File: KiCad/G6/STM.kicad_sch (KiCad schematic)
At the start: 8 parts, among them U12 STM32C051K8T6, Y1 ABS07-32.768KHZ-1-T

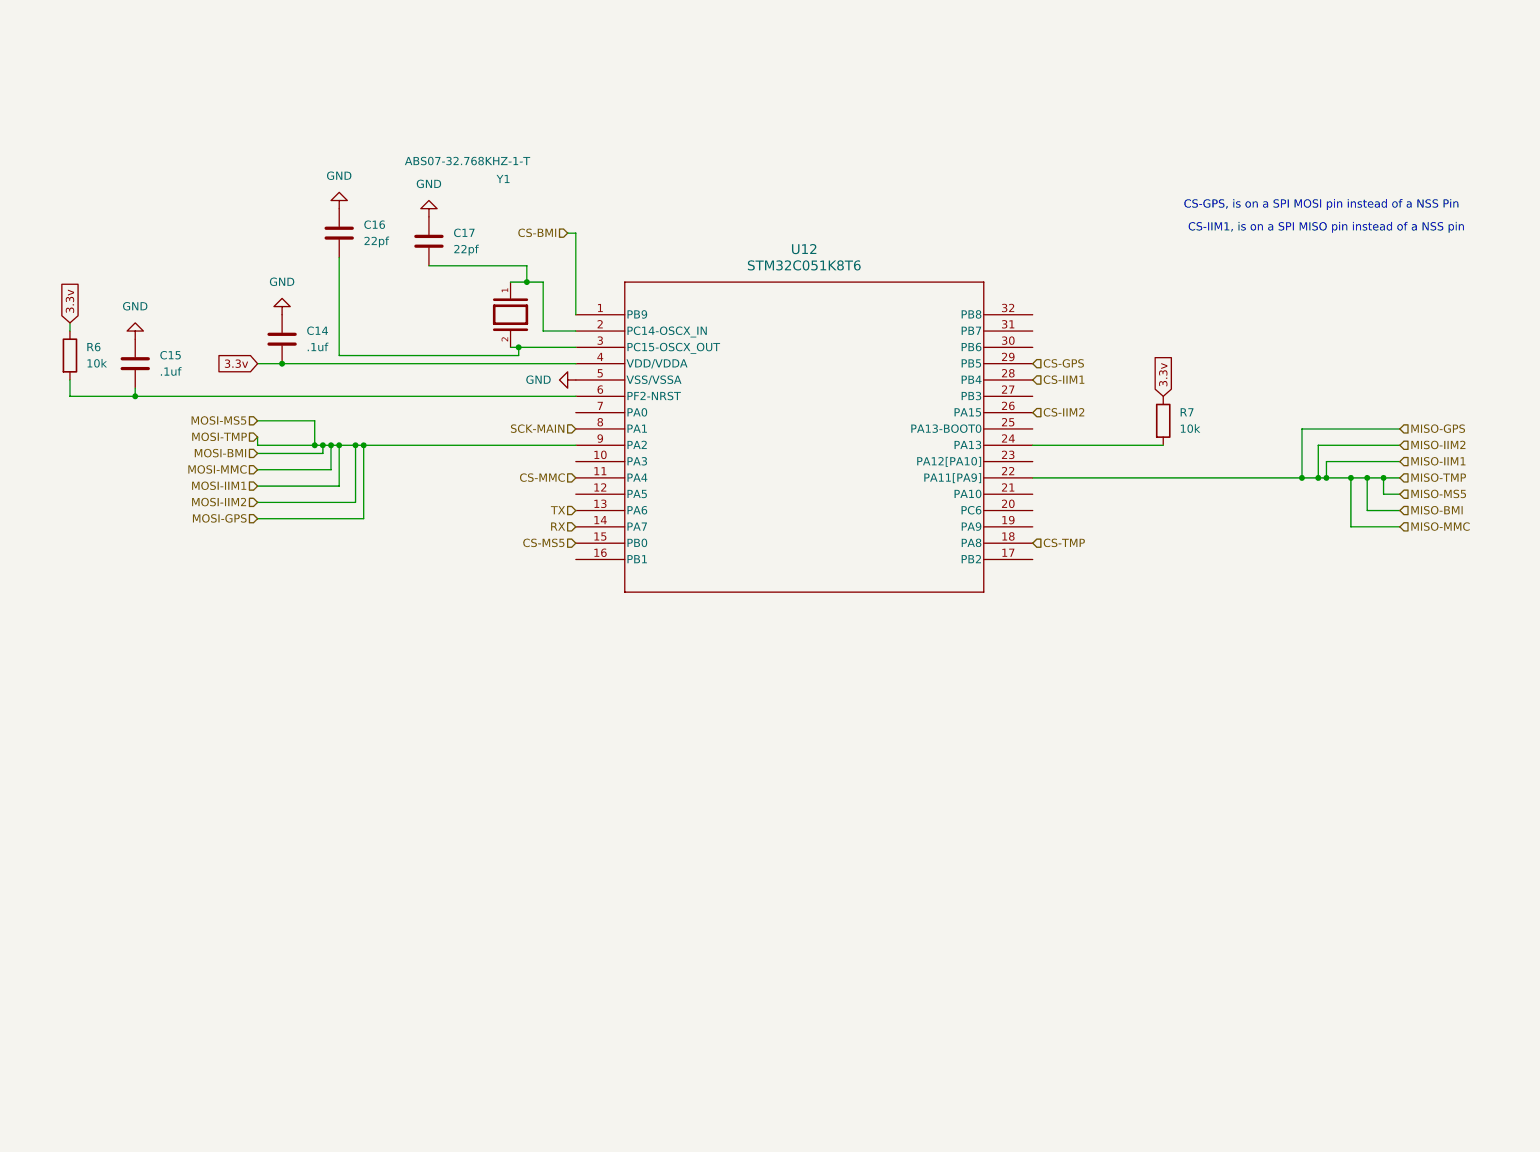
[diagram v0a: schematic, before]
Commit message: g6
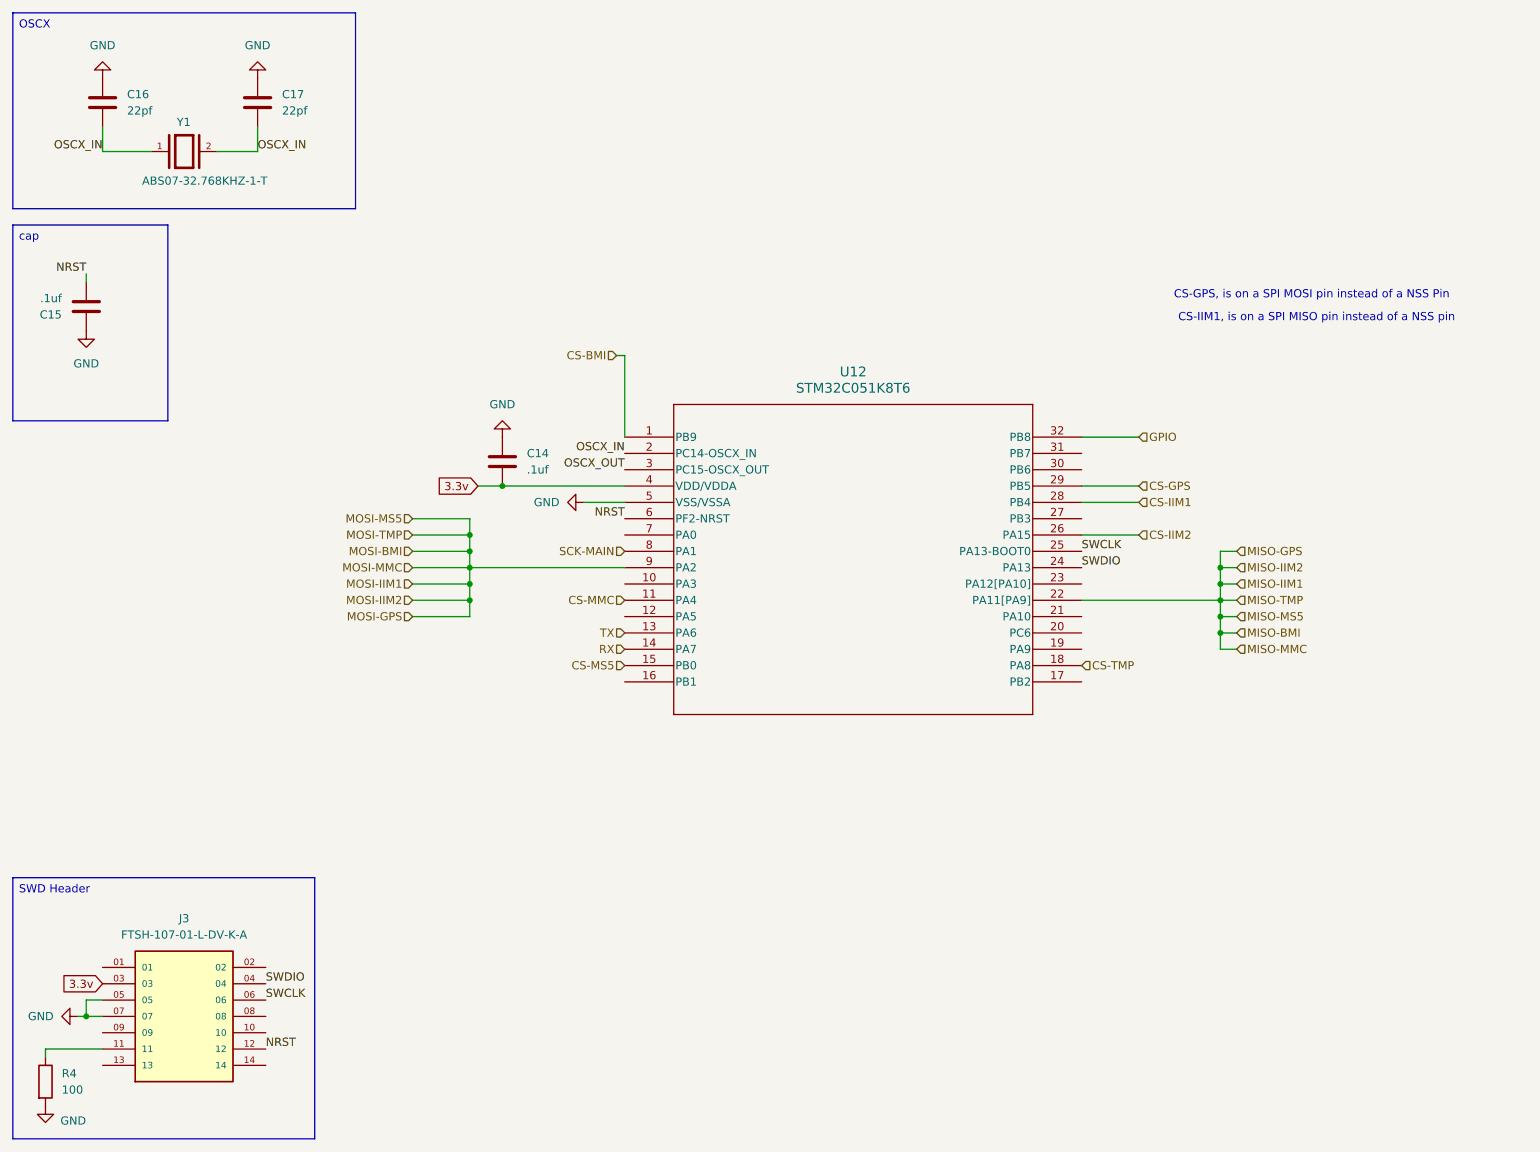
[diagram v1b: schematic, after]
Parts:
- removed R6, R7: 10k, CC0603KRXQRQBB104:10kRC1206N_YAG, symbol Device:R
- added J3: FTSH-107-01-L-DV-K-A, FTSH_107_01_L_DV_K_A:SAMTEC_FTSH-107-01-L-DV-K-A, symbol FTSH-107-01-L-DV-K-A:FTSH-107-01-L-DV-K-A
- added R4: 100, Resistor_SMD:R_0805_2012Metric, symbol Device:R
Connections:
- net 3.3v: now also J3.03
- net GND: now also J3.05, J3.07, R4.2
- net OSCX_IN: now reaches C16.2, Y1.2
- net OSCX_IN: now also C17.2, U12.2 (PC14-OSCX_IN), Y1.1; no longer U12.3 (PC15-OSCX_OUT)
- net SWDIO: now reaches U12.24 (PA13)
- net SWDIO: now also J3.04
- net SWCLK: now reaches U12.25 (PA13-BOOT0)
- net SWCLK: now also J3.06
- net GPIO: now reaches U12.32 (PB8)
- net NRST: now reaches C15.2, U12.6 (PF2-NRST)
- net NRST: now also J3.12
- new net: J3.11, R4.1
- new net OSCX_OUT: U12.3 (PC15-OSCX_OUT)
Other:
- moved on the sheet: C14, C15, C16, C17, U12, Y1
